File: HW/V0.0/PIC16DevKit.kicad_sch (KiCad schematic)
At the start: 0 parts

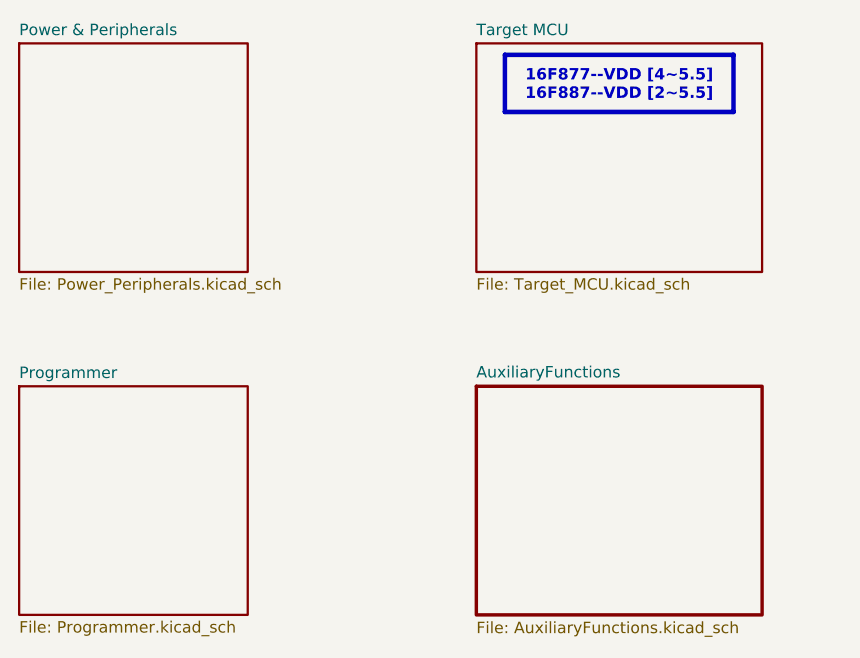
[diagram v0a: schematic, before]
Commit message: PIC16-DevKit-SCH-877 schematic update 1
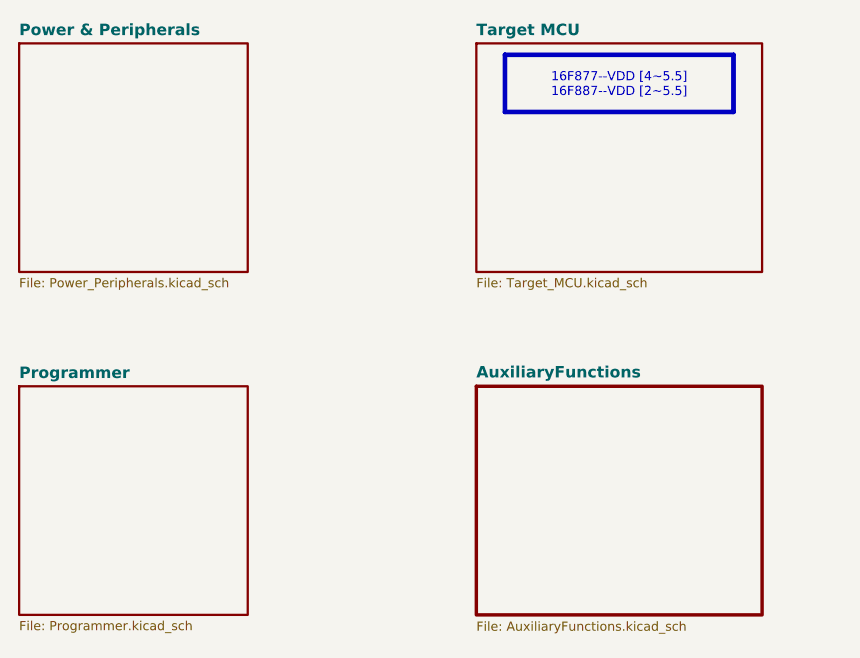
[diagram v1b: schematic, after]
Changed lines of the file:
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@@
 			(font
 				(face "Consolas")
-				(size 1.27 1.27)
+				(size 1.016 1.016)
 				(thickness 0.254)
-				(bold yes)
 			)
 		)
@@
 			(effects
 				(font
+					(face "Consolas")
 					(size 1.27 1.27)
+					(bold yes)
 				)
 				(justify left bottom)
@@
 			(effects
 				(font
-					(size 1.27 1.27)
+					(face "Consolas")
+					(size 1.016 1.016)
 				)
 				(justify left top)
@@
 			(effects
 				(font
+					(face "Consolas")
 					(size 1.27 1.27)
+					(bold yes)
 				)
 				(justify left bottom)
@@
 			(effects
 				(font
-					(size 1.27 1.27)
+					(face "Consolas")
+					(size 1.016 1.016)
 				)
 				(justify left top)
@@
 			(effects
 				(font
+					(face "Consolas")
 					(size 1.27 1.27)
+					(bold yes)
 				)
 				(justify left bottom)
@@
 			(effects
 				(font
-					(size 1.27 1.27)
+					(face "Consolas")
+					(size 1.016 1.016)
 				)
 				(justify left top)
@@
 			(effects
 				(font
+					(face "Consolas")
 					(size 1.27 1.27)
+					(bold yes)
 				)
 				(justify left bottom)
@@
 			(effects
 				(font
-					(size 1.27 1.27)
+					(face "Consolas")
+					(size 1.016 1.016)
 				)
 				(justify left top)
